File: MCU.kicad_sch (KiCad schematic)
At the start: 10 parts, among them U1 STM32U031C6Ux

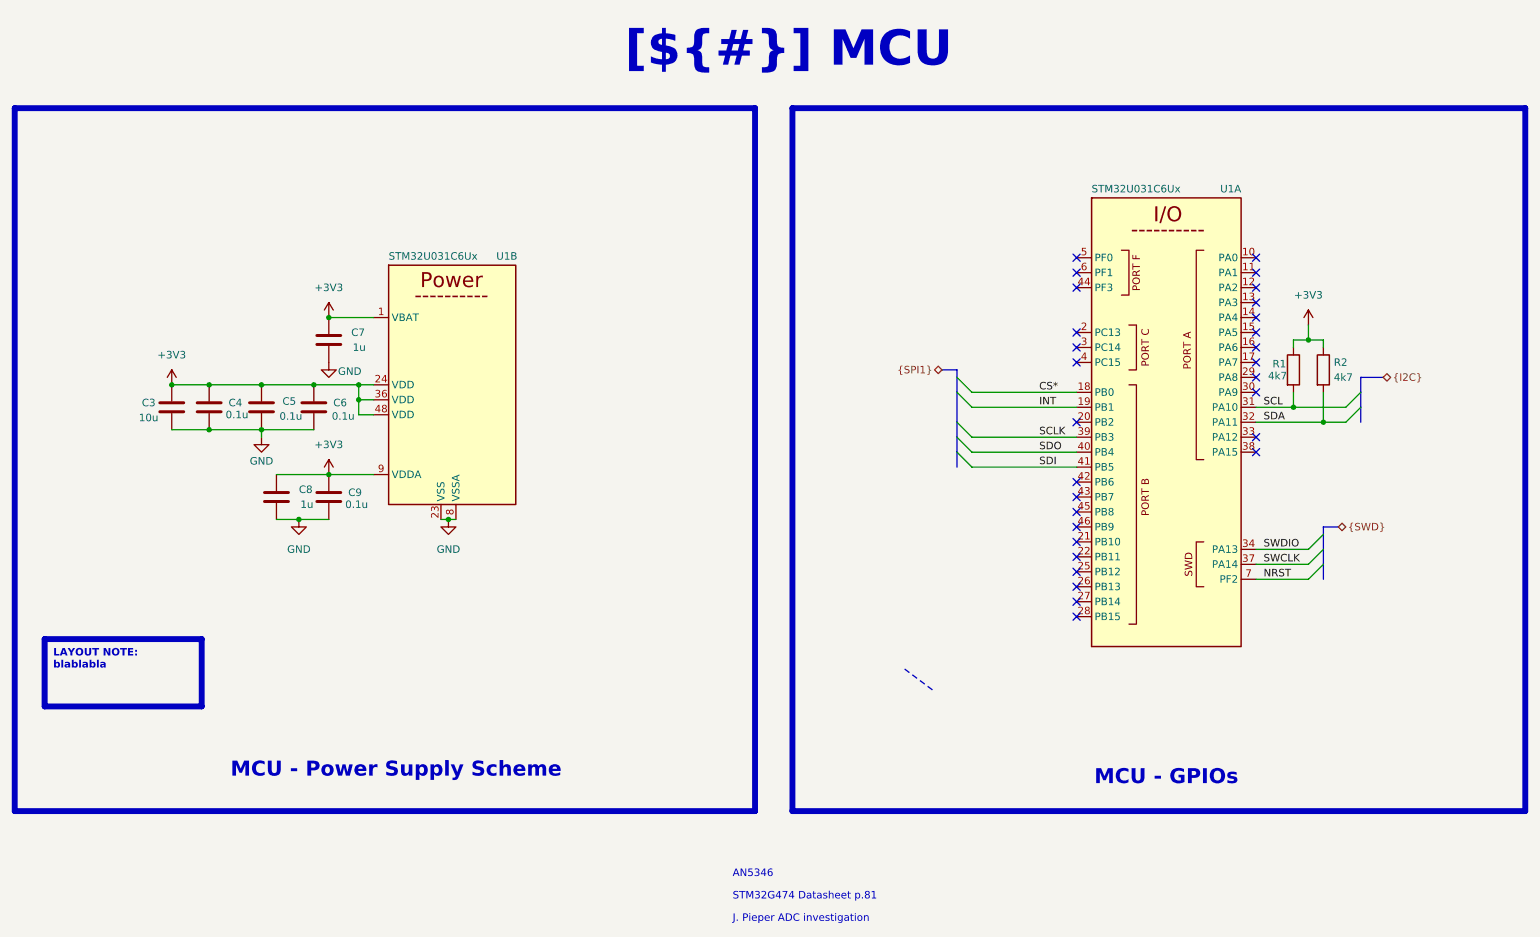
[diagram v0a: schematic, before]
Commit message: updated structure
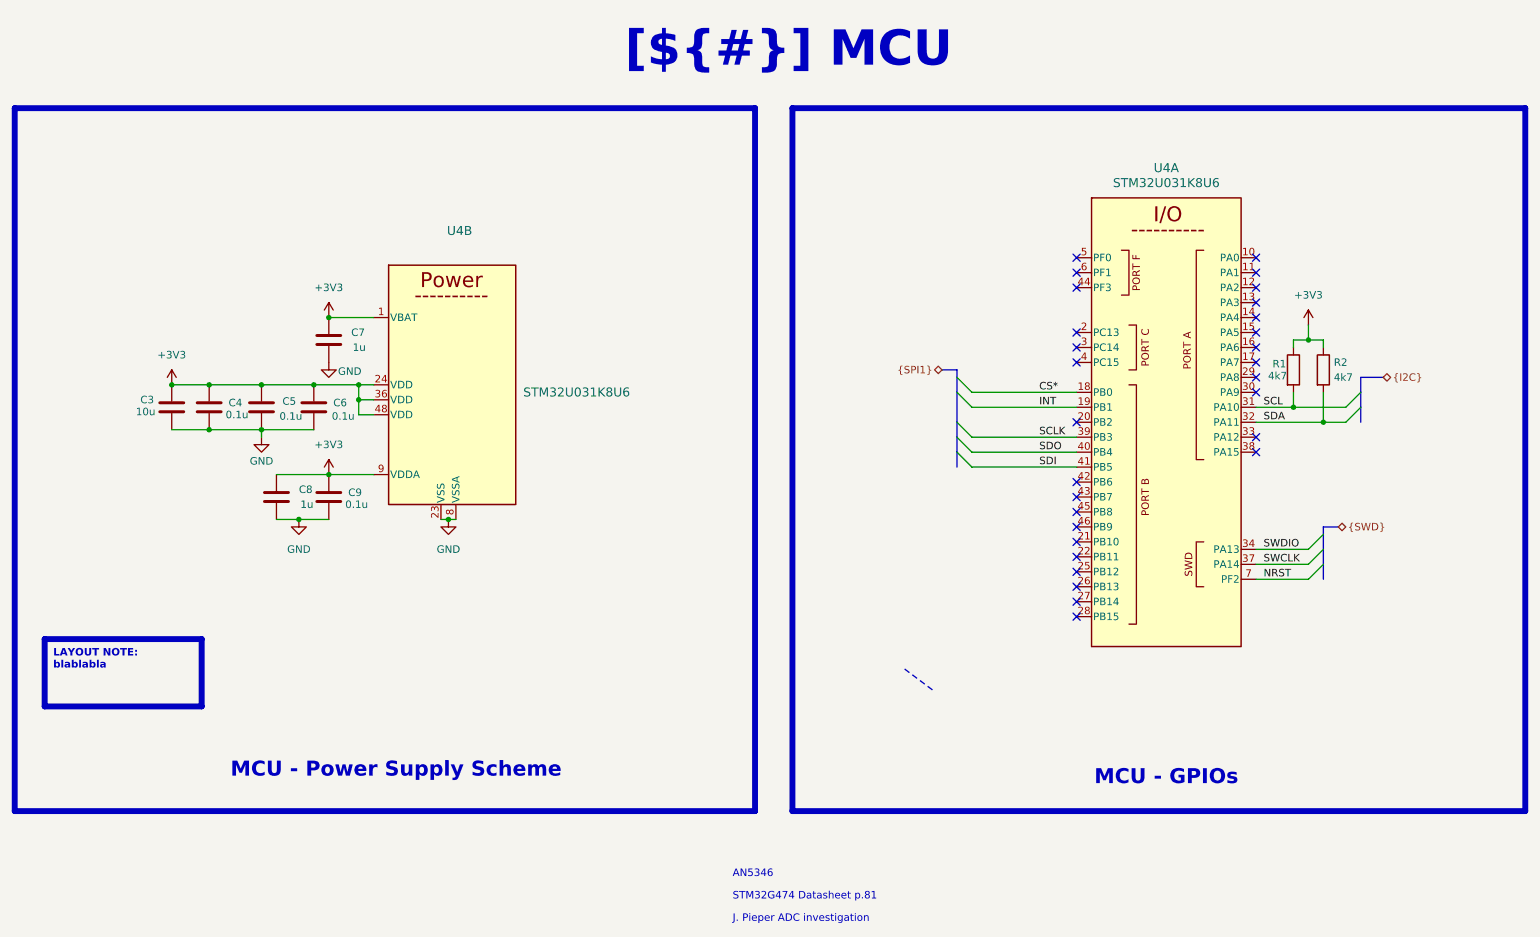
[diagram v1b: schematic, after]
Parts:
- removed U1: STM32U031C6Ux, Package_DFN_QFN:QFN-48-1EP_7x7mm_P0.5mm_EP5.6x5.6mm, symbol MCU_ST_STM32U0:STM32U031C6Ux
- added U4: STM32U031K8U6, 0_mcu:UFQFPN-32_STM, symbol 0_mcu:STM32U031K8U6
- C3: footprint (none) -> 0_capacitor_SMD:C_0603_1608Metric; Manufacturer (none) -> Samsung; Manufacturer Part Number (none) -> CL10A106KP8NNNC
- C4, C5, C6, C9: footprint (none) -> 0_capacitor_SMD:C_0402_1005Metric; Manufacturer (none) -> KEMET; Manufacturer Part Number (none) -> C0402C104K8RAC
- C7, C8: footprint (none) -> 0_capacitor_SMD:C_0603_1608Metric; Manufacturer (none) -> YAGEO; Manufacturer Part Number (none) -> CC0603KRX5R6BB105
- R1, R2: footprint (none) -> 0_resistor_SMD:R_0402_1005Metric; Manufacturer (none) -> YAGEO; Manufacturer Part Number (none) -> RC0402FR-074K7L
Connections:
- net +3V3: now also U4.1 (VBAT), U4.24 (VDD), U4.36 (VDD), U4.48 (VDD), U4.9 (VDDA)
- net CS*: now also U4.18 (PB0)
- net GND: now also U4.23 (VSS), U4.35 (VSS), U4.47 (VSS), U4.49 (VSS), U4.8 (VSSA)
- net INT: now also U4.19 (PB1)
- net NRST: now also U4.7 (PF2)
- net SCL: now also U4.31 (PA10)
- net SCLK: now also U4.39 (PB3)
- net SDA: now also U4.32 (PA11)
- net SDI: now also U4.41 (PB5)
- net SDO: now also U4.40 (PB4)
- net SWCLK: now also U4.37 (PA14)
- net SWDIO: now also U4.34 (PA13)
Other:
- title: Sheet Title A -> MCU
